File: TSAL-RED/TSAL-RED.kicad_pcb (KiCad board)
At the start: 2 copper layers, 47 parts, among them J1 Conn_01x02, J2 Conn_01x02, K1 G5V-2, Q1 2N7002, Q2 IRF9540N, U1 LM358, U2 4N35, U3 NE555D

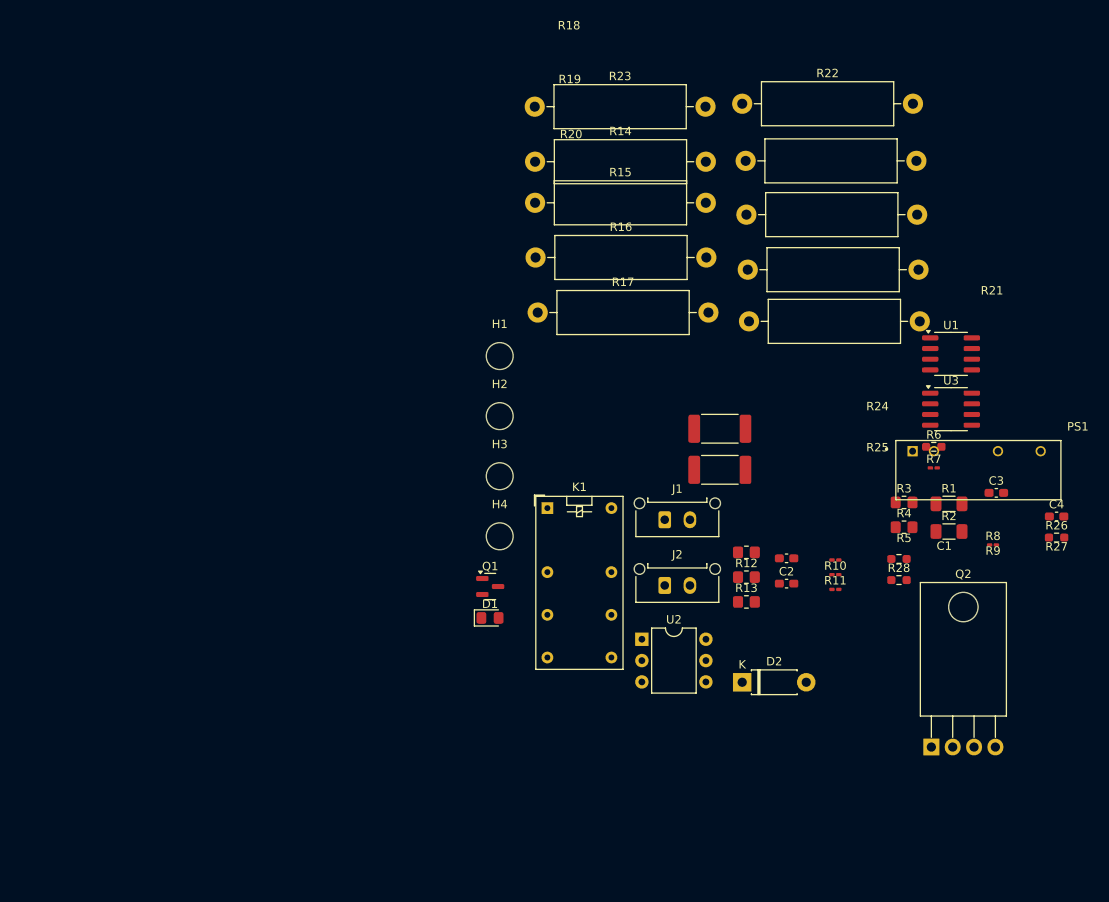
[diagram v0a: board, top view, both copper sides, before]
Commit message: CREATE TSAL PCBs
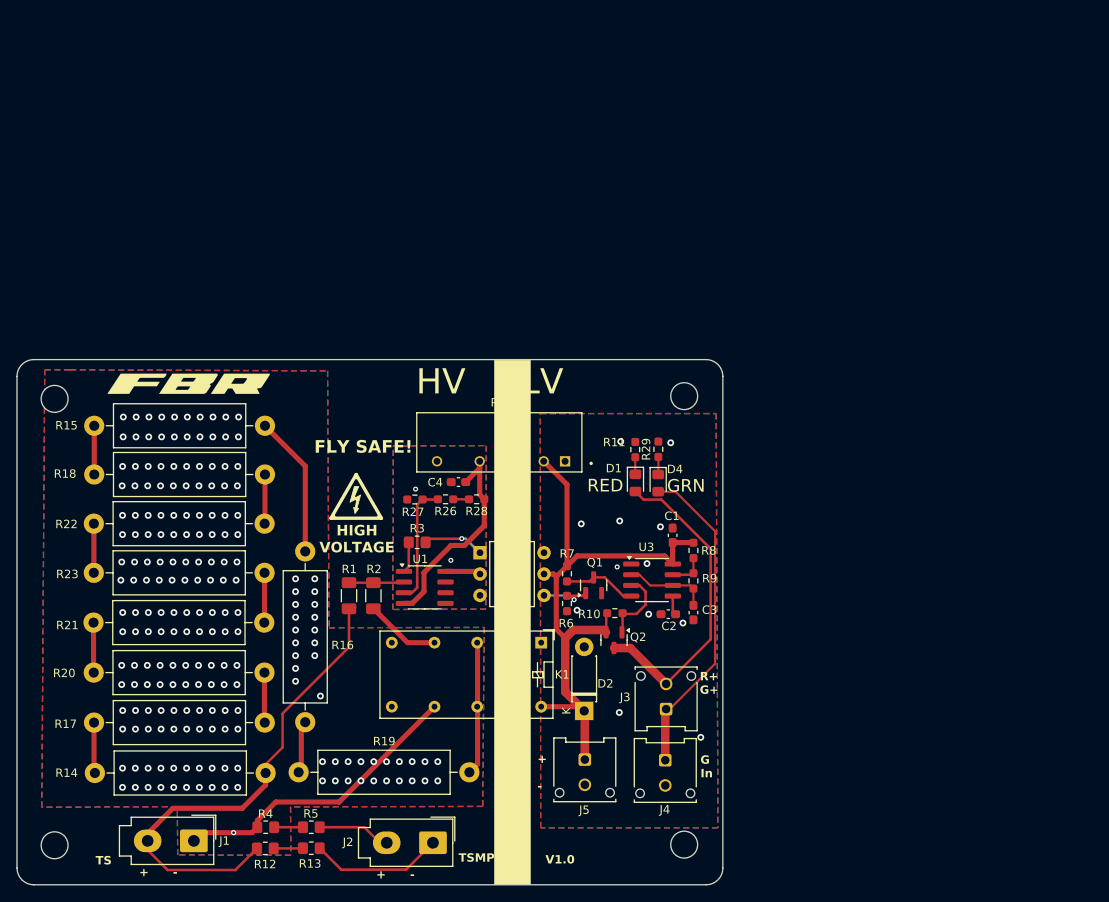
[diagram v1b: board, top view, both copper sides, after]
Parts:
- removed R24, R25: 100, Resistor_SMD:R_2512_6332Metric_Pad1.40x3.35mm_HandSolder
- added D4: GRN, LED_SMD:LED_0805_2012Metric_Pad1.15x1.40mm_HandSolder, F.Cu at (126.1, 74.5)
- added G***: LOGO, LOGO, F.Cu at (70.0, 62.6)
- added J3: Conn_02x01, Connector_Molex:Molex_Micro-Fit_3.0_43045-0212_2x01_P3.00mm_Vertical, F.Cu at (127.0, 101.4)
- added J4: Conn_02x01, Connector_Molex:Molex_Micro-Fit_3.0_43045-0212_2x01_P3.00mm_Vertical, F.Cu at (126.9, 107.5)
- added J5: Conn_02x01, Connector_Molex:Molex_Micro-Fit_3.0_43045-0212_2x01_P3.00mm_Vertical, F.Cu at (117.3, 107.4)
- added R29: 2k2, Resistor_SMD:R_0603_1608Metric_Pad0.98x0.95mm_HandSolder, F.Cu at (126.1, 70.5)
- added REF**: Symbol_HighVoltage_Triangle_6x6mm_Copper, Symbol:Symbol_HighVoltage_Triangle_6x6mm_Copper, F.Cu at (90.1, 76.1)
- J1, J2: footprint Connector_Molex:Molex_Micro-Fit_3.0_43650-0215_1x02_P3.00mm_Vertical -> Connector_Molex:Molex_Mini-Fit_Jr_5566-02A_2x01_P4.20mm_Vertical
- Q2: value IRF9540N -> AO3401A; footprint Package_TO_SOT_THT:TO-220-4_Horizontal_TabDown -> Package_TO_SOT_SMD:SOT-23
- R10, R11, R7, R8, R9: footprint Resistor_SMD:R_0201_0603Metric_Pad0.64x0.40mm_HandSolder -> Resistor_SMD:R_0603_1608Metric_Pad0.98x0.95mm_HandSolder
- R28: value 330 -> 910
- moved R18 86.0 mm to (59.0, 73.5)
- moved R21 85.9 mm to (58.9, 91.1)
- moved R19 85.1 mm to (83.3, 108.9)
- moved R4 83.9 mm to (79.4, 115.5)
- moved R14 79.5 mm to (79.4, 109.0), turned to 180 degrees
- moved R23 76.4 mm to (58.9, 85.2)
- moved R22 75.7 mm to (79.2, 79.3), turned to 180 degrees
- moved R20 74.9 mm to (79.2, 97.0), turned to 180 degrees
- moved H2 73.6 mm to (54.2, 117.6)
- moved R26 72.9 mm to (100.8, 76.4), turned to 180 degrees
- moved R1 72.2 mm to (89.3, 87.9), turned to -90 degrees
- moved R17 71.9 mm to (58.9, 103.0)
- moved C4 71.3 mm to (102.3, 74.4), turned to 180 degrees
- moved R2 68.9 mm to (92.2, 87.9), turned to -90 degrees
- moved U1 68.5 mm to (98.3, 86.9)
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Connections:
- U1 pad 2: /Vref -> /Vin
- U1 pad 3: /Vin -> /Vref
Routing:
- net GLV+: track 0.00 -> 72.0 mm
- net TS+: track 0.00 -> 59.2 mm
- net TS-: track 0.00 -> 44.8 mm, vias 0 -> 198
- net /GRN+: track 0.00 -> 38.7 mm
- net /RED+: track 0.00 -> 38.5 mm
- net /5V+_Iso: track 0.00 -> 25.9 mm
- net Net-(R15-Pad2): track 0.00 -> 16.9 mm
- net Net-(J2-Pin_1): track 0.00 -> 15.9 mm
- net Net-(K1-Pad13): track 0.00 -> 15.4 mm
- net /Vref: track 0.00 -> 14.4 mm
- net Net-(U3-THR): track 0.00 -> 10.1 mm
- net Net-(J2-Pin_2): track 0.00 -> 9.66 mm
- net Net-(Q2-G): track 0.00 -> 9.38 mm
- net Net-(Q1-D): track 0.00 -> 8.77 mm
- net Net-(R3-Pad2): track 0.00 -> 7.35 mm, vias 0 -> 1
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- added copper zone on B.Cu, net /5V-_Iso
- added copper zone on F.Cu, net /5V-_Iso
- added copper zone on B.Cu, net GLV-
- added copper zone on F.Cu, net GLV-
- added copper zone on B.Cu, net TS-
- added copper zone on F.Cu, net TS-
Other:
- board outline added: 84 x 62.5 mm
- board text added: "+ -"
- board text added: "0.2000 mm / 0.2000 mm"
- board text added: "0.3000 mm"
- board text added: "1.6000 mm"
- board text added: "2"
- board text added: "84.0000 mm x 62.5000 mm"
- board text added: "BOARD CHARACTERISTICS"
- board text added: "Board Thickness:"
- board text added: "Board overall dimensions:"
- board text added: "Castellated pads:"
- board text added: "Copper Finish:"
- board text added: "Copper Layer Count:"
- board text added: "Edge card connectors:"
- board text added: "FLY SAFE!"
- board text added: "G In"
- board text added: "GRN"
- board text added: "HAL SnPb"
- board text added: "HIGH VOLTAGE"
- board text added: "HV LV"
- board text added: "Impedance Control:"
- board text added: "Min hole diameter:"
- board text added: "Min track/spacing:"
- board text added: "No"
- board text added: "Plated Board Edge:"
- board text added: "R+ G+"
- board text added: "RED"
- board text added: "TS"
- board text added: "TSMP"
- board text added: "V1.0"
